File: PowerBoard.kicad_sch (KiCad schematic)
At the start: 50 parts

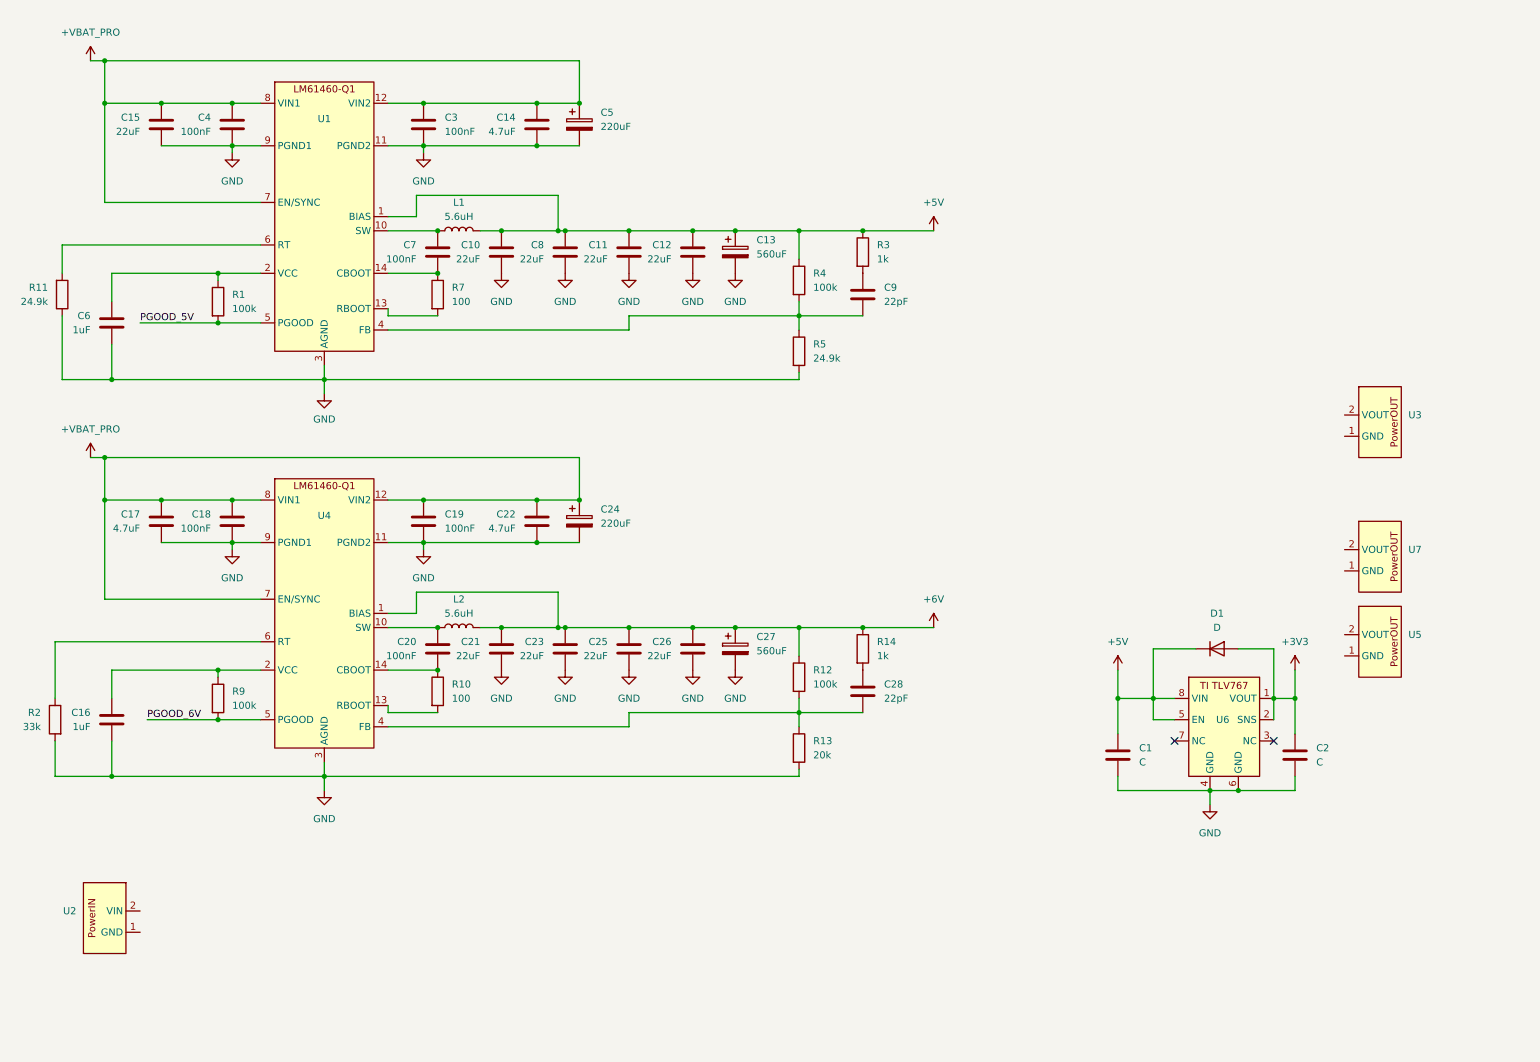
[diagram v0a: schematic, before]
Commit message: finished schematic
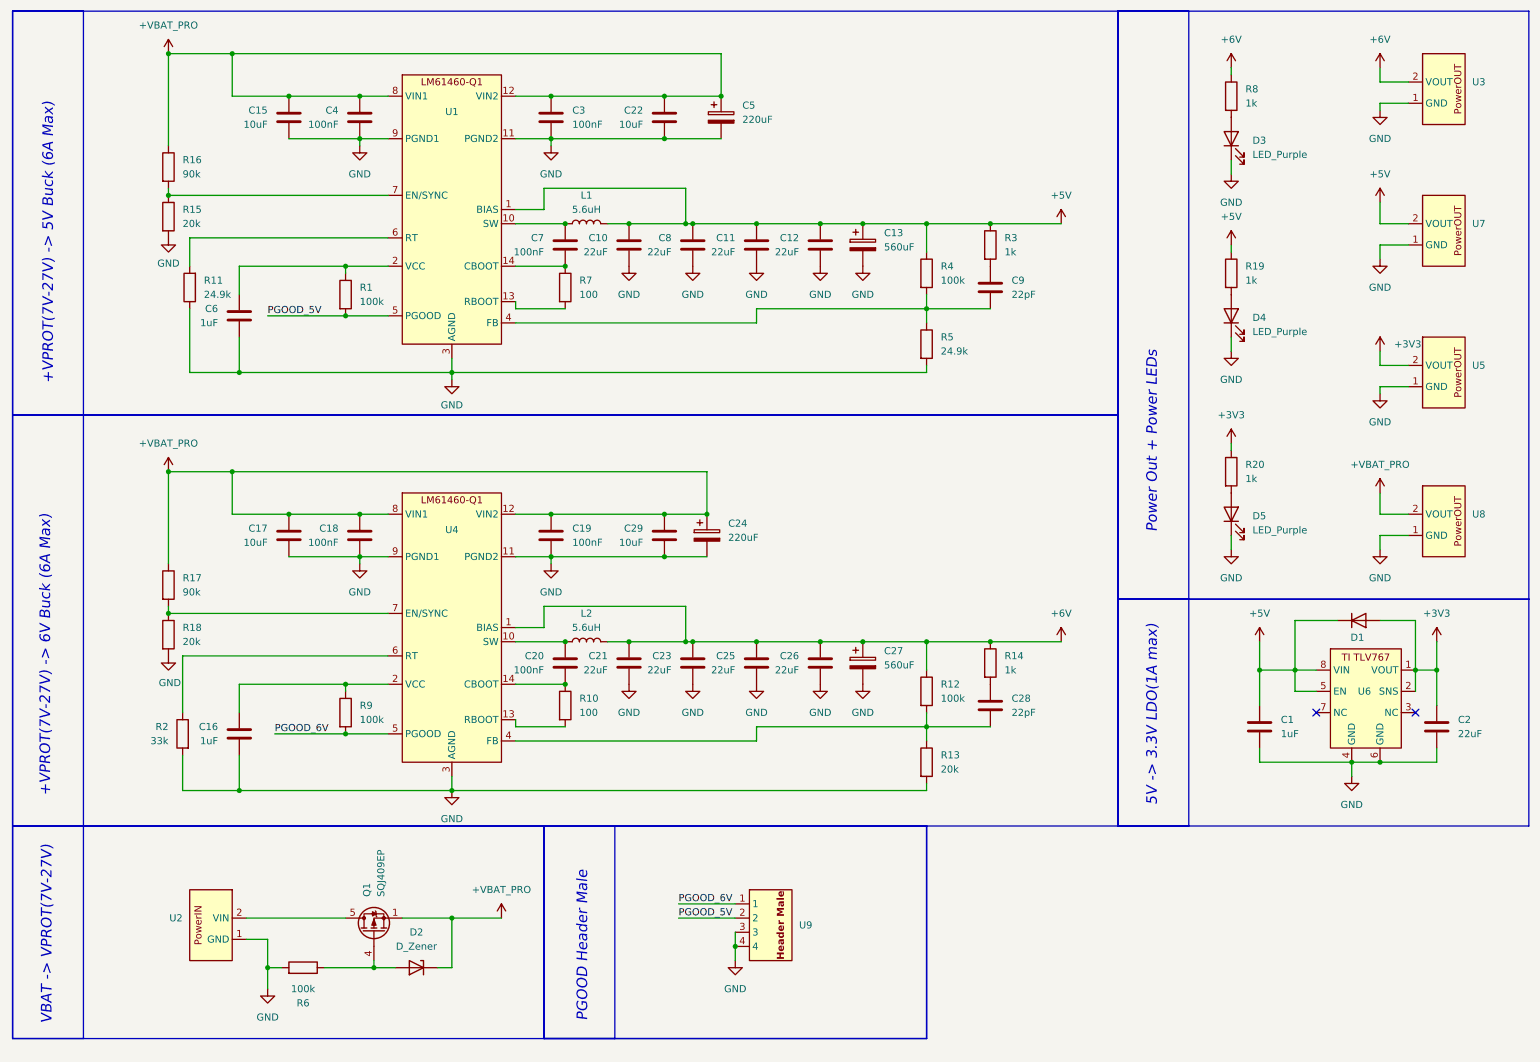
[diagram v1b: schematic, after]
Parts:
- removed C14: 4.7uF, symbol Device:C
- added C29: 10uF, Capacitor_SMD:C_1206_3216Metric, symbol Device:C
- added D2: D_Zener, Package_TO_SOT_SMD:SOT-23, symbol Device:D_Zener
- added D3, D4, D5: LED_Purple, symbol Device:LED
- added Q1: SQJ409EP, Package_SO:PowerPAK_SO-8L_Single, symbol Transistor_FET:SQJ409EP
- added R15, R18: 20k, Resistor_SMD:R_0603_1608Metric, symbol Device:R
- added R16, R17: 90k, Resistor_SMD:R_0603_1608Metric, symbol Device:R
- added R19, R20, R8: 1k, Resistor_SMD:R_0603_1608Metric, symbol Device:R
- added R6: 100k, Resistor_SMD:R_0603_1608Metric, symbol Device:R
- added U8: (no value), symbol PowerBoard:PowerOutput
- added U9: (no value), symbol powerBoardSchool:4x1_Header_Male
- C1: value C -> 1uF; footprint (none) -> Capacitor_SMD:C_0603_1608Metric
- C10, C11, C12, C21, C23, C25, C26, C8: footprint (none) -> Capacitor_SMD:C_1210_3225Metric
- C13, C24, C27, C5: footprint (none) -> Capacitor_SMD:CP_Elec_8x10.5
- C15: value 22uF -> 10uF; footprint (none) -> Capacitor_SMD:C_1206_3216Metric
- C16, C18, C19, C20, C28, C3, C4, C6, C7, C9: footprint (none) -> Capacitor_SMD:C_0603_1608Metric
- C17, C22: value 4.7uF -> 10uF; footprint (none) -> Capacitor_SMD:C_1206_3216Metric
- C2: value C -> 22uF; footprint (none) -> Capacitor_SMD:C_1210_3225Metric
- D1: footprint (none) -> Diode_SMD:D_SMA
- R1, R10, R11, R12, R13, R14, R2, R3, R4, R5, R7, R9: footprint (none) -> Resistor_SMD:R_0603_1608Metric
- U1, U2, U3, U4, U5, U6, U7: value ~ -> (none)
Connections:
- net +3V3: now also U5.2 (VOUT), R20.1
- net +5V: now also U7.2 (VOUT), R19.1
- net +6V: now also U3.2 (VOUT), R8.1
- net +VBAT_PRO: now also C29.1, D2.1 (K), Q1.1 (S), Q1.2 (S), Q1.3 (S), R16.1, R17.1, U8.2 (VOUT); no longer U1.7 (EN/SYNC), U4.7 (EN/SYNC)
- net GND: now also U2.1 (GND), U3.1 (GND), U5.1 (GND), U7.1 (GND), C29.2, D3.1 (K), D4.1 (K), D5.1 (K), R15.2, R18.2, R6.2, U8.1 (GND), U9.3, U9.4
- net PGOOD_5V: now also U9.2
- net PGOOD_6V: now also U9.1
- net at U2.2 (VIN): now also Q1.5 (D)
- new net: D5.2 (A), R20.2
- new net: D2.2 (A), Q1.4 (G), R6.1
- new net: R15.1, R16.2, U1.7 (EN/SYNC)
- new net: D3.2 (A), R8.2
- new net: D4.2 (A), R19.2
- new net: R17.2, R18.1, U4.7 (EN/SYNC)
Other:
- note added: "+VPROT(7V-27V) -> 5V Buck (6A Max)"
- note added: "+VPROT(7V-27V) -> 6V Buck (6A Max)"
- note added: "5V -> 3.3V LDO(1A max)"
- note added: "PGOOD Header Male"
- note added: "Power Out + Power LEDs"
- note added: "VBAT -> VPROT(7V-27V)"
- moved on the sheet: C1, C10, C11, C12, C13, C15, C16, C17, C18, C19, C2, C20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
